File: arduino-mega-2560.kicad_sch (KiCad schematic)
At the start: 47 parts, among them J1 USB_B, J10 Conn_02x18_Odd_Even, J11 Conn_01x08, J4 Conn_01x08, J5 Conn_01x08, J6 Conn_01x08, J7 Conn_01x10, J8 Conn_PIC_ICSP_ICD, J9 Conn_01x08, SW1 SW_Push, U1 MCU-ATMEGA2560-16AU_TQFP100_, U2 AMS1117-5.0, U3 ATmega16U2-A, U4 25CSM04xxMF, U5 LMV358, U6 LP2985-3.3, U7 L7805, Y1 Crystal

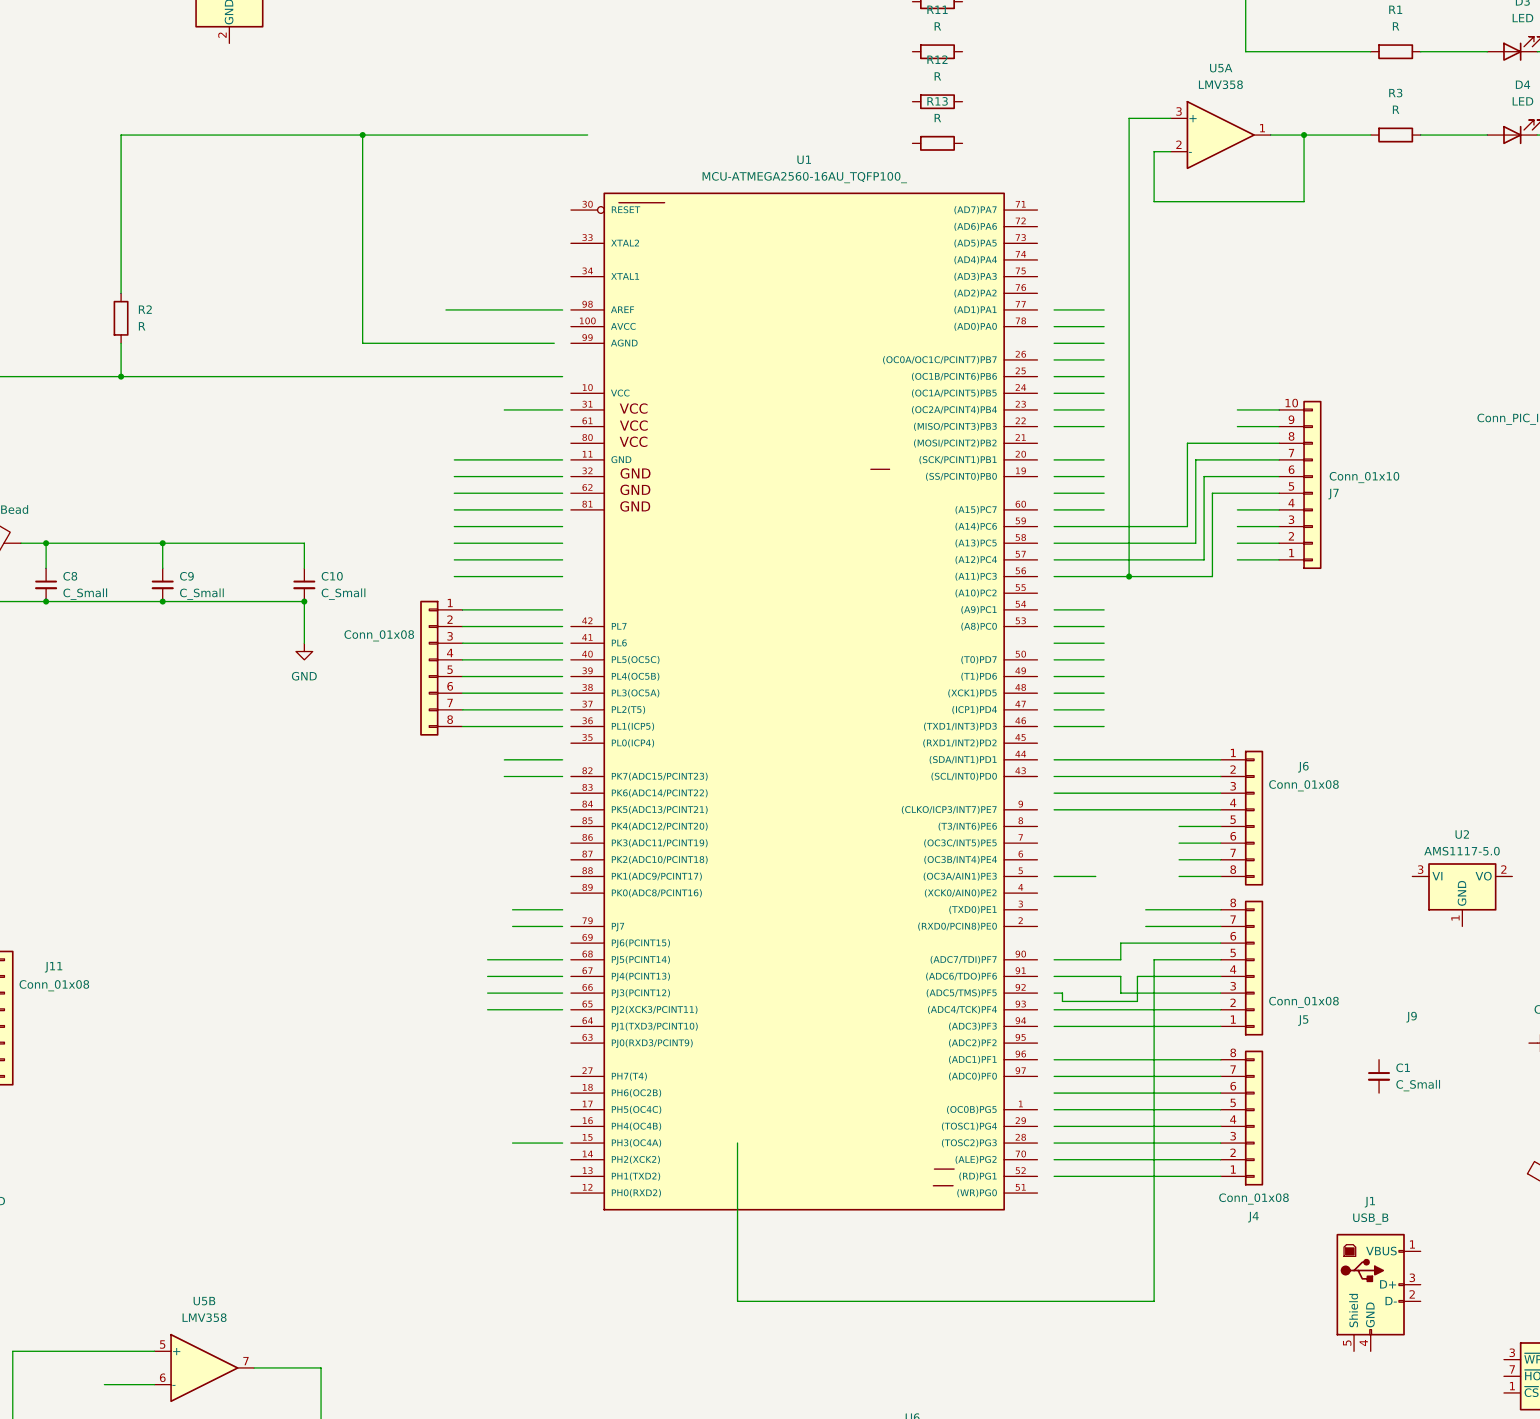
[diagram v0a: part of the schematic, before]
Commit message: updated schematic project
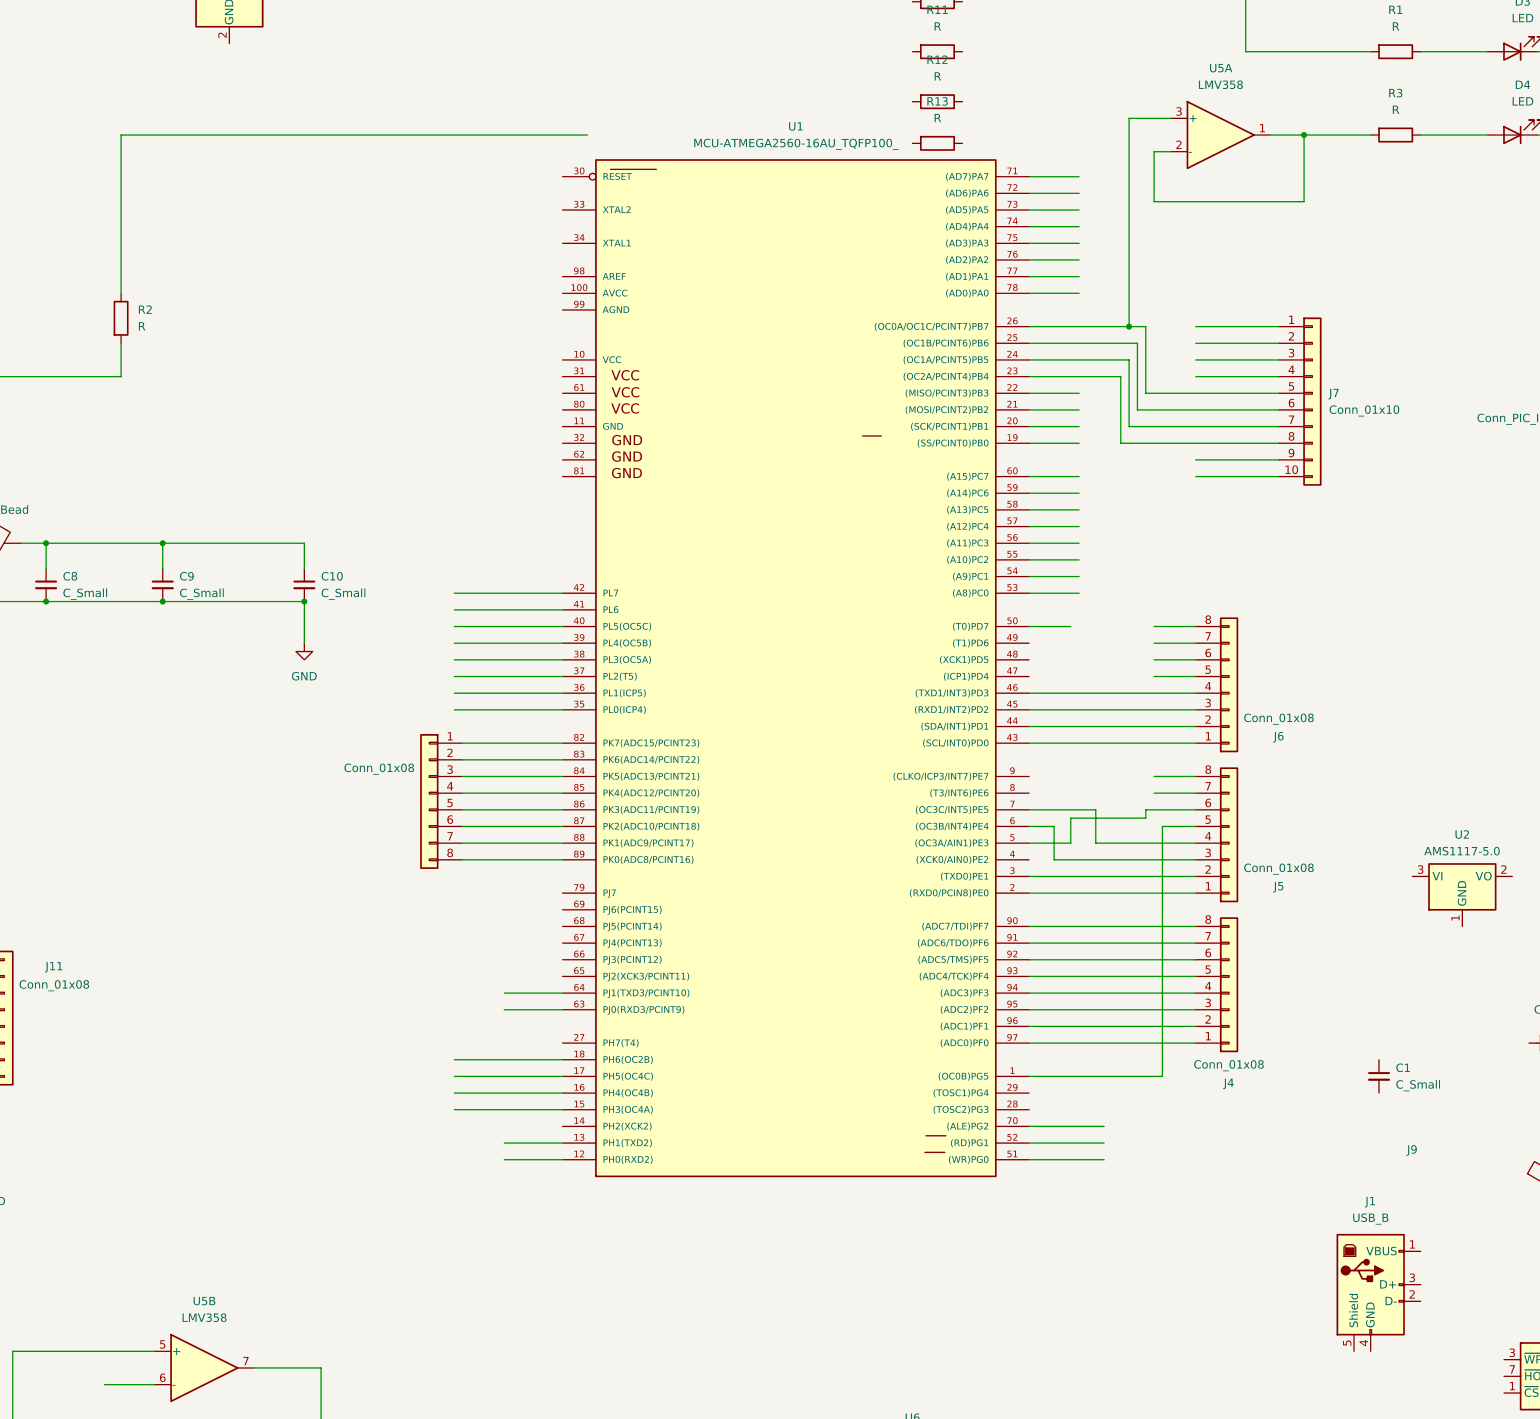
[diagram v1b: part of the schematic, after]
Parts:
- removed U1: MCU-ATMEGA2560-16AU_TQFP100_, MCU-ATMEGA2560-16AU_TQFP100_:TQFP100-0.5-14X14MM, symbol MCU-ATMEGA2560-16AU_SNAPMAGIC:MCU-ATMEGA2560-16AU_TQFP100_
- added U1: MCU-ATMEGA2560-16AU_TQFP100_, MCU-ATMEGA2560-16AU_TQFP100_:TQFP100-0.5-14X14MM, symbol MCU-ATMEGA2560-16AU_TQFP100_:MCU-ATMEGA2560-16AU_TQFP100_
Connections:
- net at J9.1 (Pin_1): now also U1.82 (PK7(ADC15/PCINT23))
- net at J9.2 (Pin_2): now also U1.83 (PK6(ADC14/PCINT22))
- net at J9.3 (Pin_3): now also U1.84 (PK5(ADC13/PCINT21))
- net at J9.4 (Pin_4): now also U1.85 (PK4(ADC12/PCINT20))
- net at J9.5 (Pin_5): now also U1.86 (PK3(ADC11/PCINT19))
- net at J9.6 (Pin_6): now also U1.87 (PK2(ADC10/PCINT18))
- net at J9.7 (Pin_7): now also U1.88 (PK1(ADC9/PCINT17))
- net at J9.8 (Pin_8): now also U1.89 (PK0(ADC8/PCINT16))
- net at J7.5 (Pin_5), U5.3 (+): now also U1.26 ((OC0A/OC1C/PCINT7)PB7)
- net at J4.1 (Pin_1): now also U1.97 ((ADC0)PF0)
- net at J4.2 (Pin_2): now also U1.96 ((ADC1)PF1)
- net at J4.3 (Pin_3): now also U1.95 ((ADC2)PF2)
- net at J4.4 (Pin_4): now also U1.94 ((ADC3)PF3)
- net at J4.5 (Pin_5): now also U1.93 ((ADC4/TCK)PF4)
- net at J4.6 (Pin_6): now also U1.92 ((ADC5/TMS)PF5)
- net at J4.7 (Pin_7): now also U1.91 ((ADC6/TDO)PF6)
- net at J4.8 (Pin_8): now also U1.90 ((ADC7/TDI)PF7)
- net at J7.6 (Pin_6): now also U1.25 ((OC1B/PCINT6)PB6)
- net at J7.7 (Pin_7): now also U1.24 ((OC1A/PCINT5)PB5)
- net at J7.8 (Pin_8): now also U1.23 ((OC2A/PCINT4)PB4)
- net at J5.1 (Pin_1): now also U1.2 ((RXD0/PCIN8)PE0)
- net at J5.2 (Pin_2): now also U1.3 ((TXD0)PE1)
- net at J5.3 (Pin_3): now also U1.6 ((OC3B/INT4)PE4)
- net at J5.4 (Pin_4): now also U1.7 ((OC3C/INT5)PE5)
- net at J5.5 (Pin_5): now also U1.1 ((OC0B)PG5)
- net at J5.6 (Pin_6): now also U1.5 ((OC3A/AIN1)PE3)
- net at J6.1 (Pin_1): now also U1.43 ((SCL/INT0)PD0)
- net at J6.2 (Pin_2): now also U1.44 ((SDA/INT1)PD1)
- net at J6.3 (Pin_3): now also U1.45 ((RXD1/INT2)PD2)
- net at J6.4 (Pin_4): now also U1.46 ((TXD1/INT3)PD3)
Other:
- moved on the sheet: J4, J5, J6, J7, J9
